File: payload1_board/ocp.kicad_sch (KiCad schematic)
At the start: 11 parts, among them Q2 SSM6K403TU_LF, U6 LTC4361HTS8-2-TRMPBF

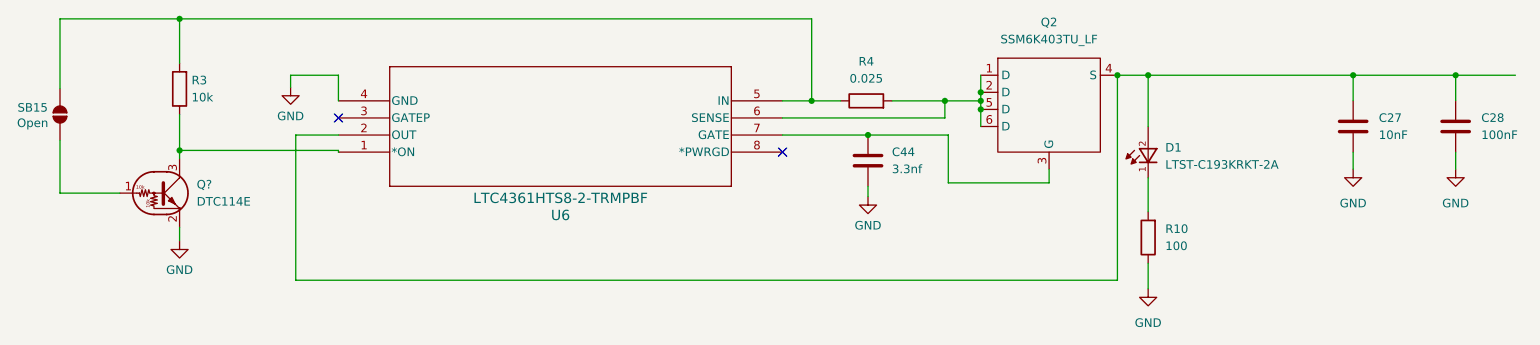
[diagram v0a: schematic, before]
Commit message: a
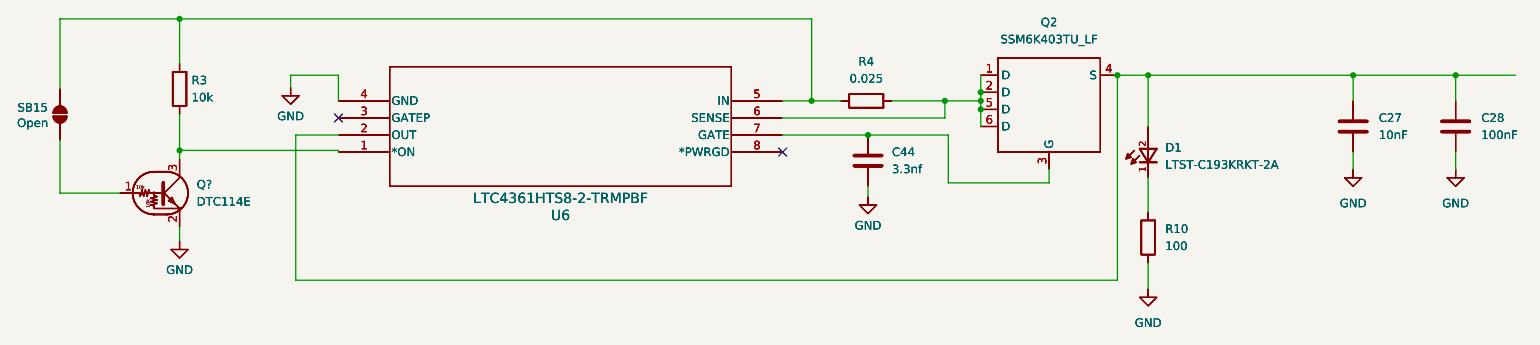
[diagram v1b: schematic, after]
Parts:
- added C27: 10nF, Capacitor_SMD:C_0805_2012Metric, symbol Device:C
- added C28: 100nF, Capacitor_SMD:C_0805_2012Metric, symbol Device:C
- added C44: 3.3nf, symbol Device:C
- added D1: LTST-C193KRKT-2A, LTST-C193KRKT-2A:0603, symbol LTST-C193KRKT-2A:LTST-C193KRKT-2A
- added Q2: SSM6K403TU_LF, SSM6K403TU_LF:UF6_TOS-L, symbol SSM6K403TU_LF:SSM6K403TU_LF
- added Q?: DTC114E, symbol Transistor_BJT:DTC114E
- added R10: 100, Resistor_SMD:R_0805_2012Metric, symbol Device:R
- added R3: 10k, symbol Device:R
- added R4: 0.025, symbol Device:R
- added SB15: Open, symbol Jumper:SolderJumper_2_Open
- added U6: LTC4361HTS8-2-TRMPBF, TSOT-23_TS8_LIT, symbol 2024-08-14_17-14-28:LTC4361HTS8-2-TRMPBF
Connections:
- net GND: now also C27.2, C28.2, C44.1, Q?.2 (E), R10.1, U6.4 (GND)
- net at Q2.1 (D), Q2.2 (D), Q2.5 (D)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: now also Q2.1 (D), Q2.2 (D), Q2.5 (D), Q2.6 (D), R4.2, U6.6 (SENSE)
- net at C44.2, Q2.3 (G), U6.7 (GATE): now also C44.2, Q2.3 (G), U6.7 (GATE)
- net at C27.1, C28.1, D1.2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: now also C27.1, C28.1, D1.2, Q2.4 (S), U6.2 (OUT)
- net at Q?.1 (B), SB15.1 (A): now also Q?.1 (B), SB15.1 (A)
- net at R3.2, R4.1, SB15.2 (B)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: now also R3.2, R4.1, SB15.2 (B), U6.5 (IN)
- net at D1.1, R10.2: now also D1.1, R10.2
- net at Q?.3 (C), R3.1, U6.1 (*ON): now also Q?.3 (C), R3.1, U6.1 (*ON)
- net at U6.3 (GATEP): now also U6.3 (GATEP)
- net at U6.8 (*PWRGD): now also U6.8 (*PWRGD)
